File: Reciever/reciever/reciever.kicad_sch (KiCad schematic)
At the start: 24 parts, among them J1 USB_C_Receptacle_USB2.0_14P, J2 UART/I2C, J3 TWAI, SW1 Button, SW2 Button, U1 TXS0102DCU, U2 LM66200, U3 SE5218ALG-LF, U4 ESP32-C6-MINI-1, U5 TCAN330DR

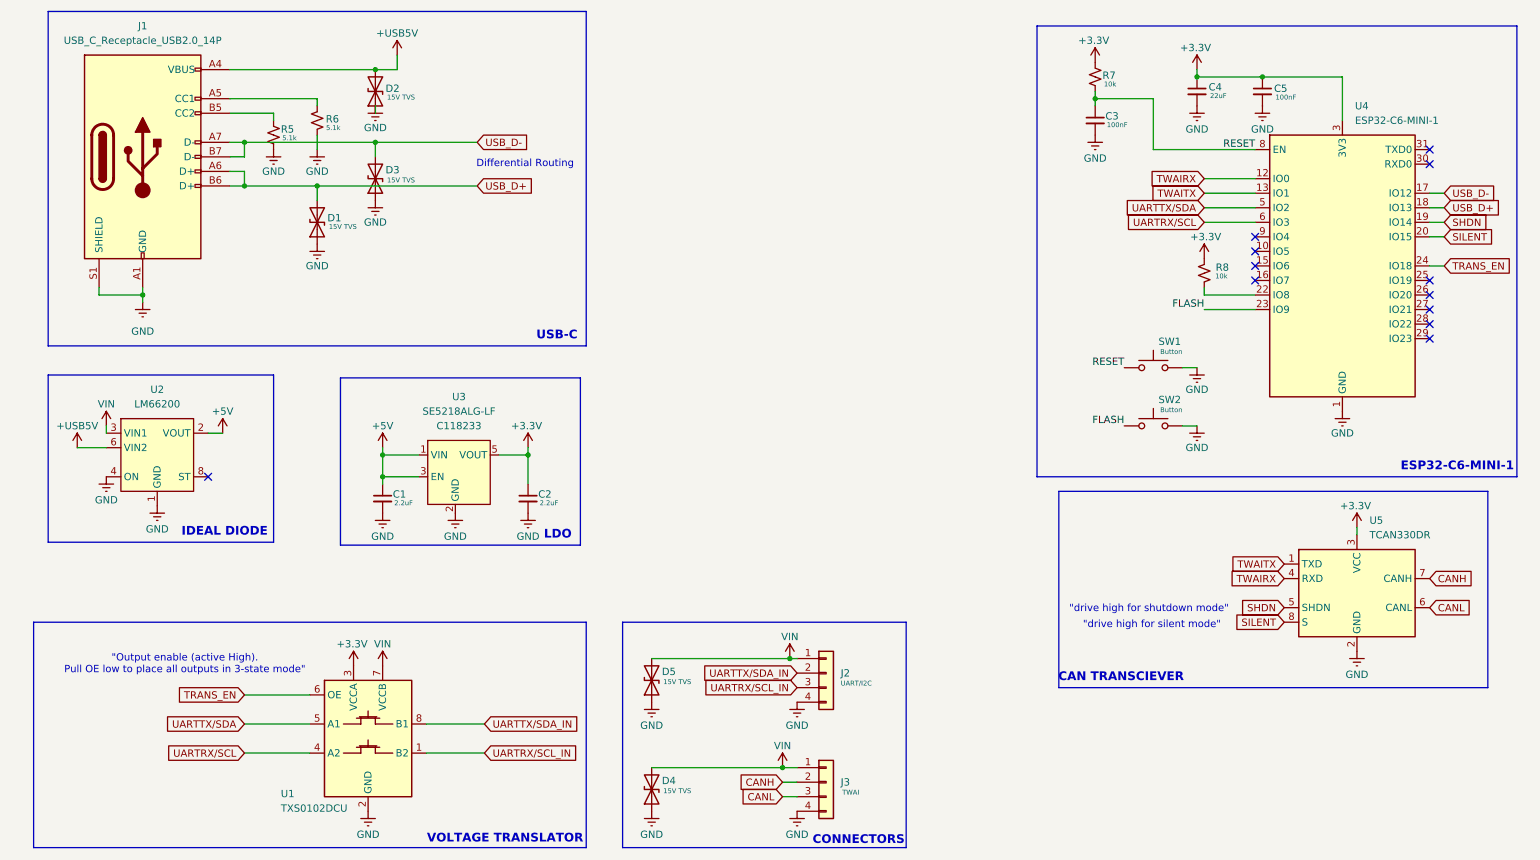
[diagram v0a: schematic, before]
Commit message: Custom RC V2
Final Remote + Receiver!

Special thanks to the CRCW25 Electrical Team who contributed to its development!

Jun
Katie
Nelson
David
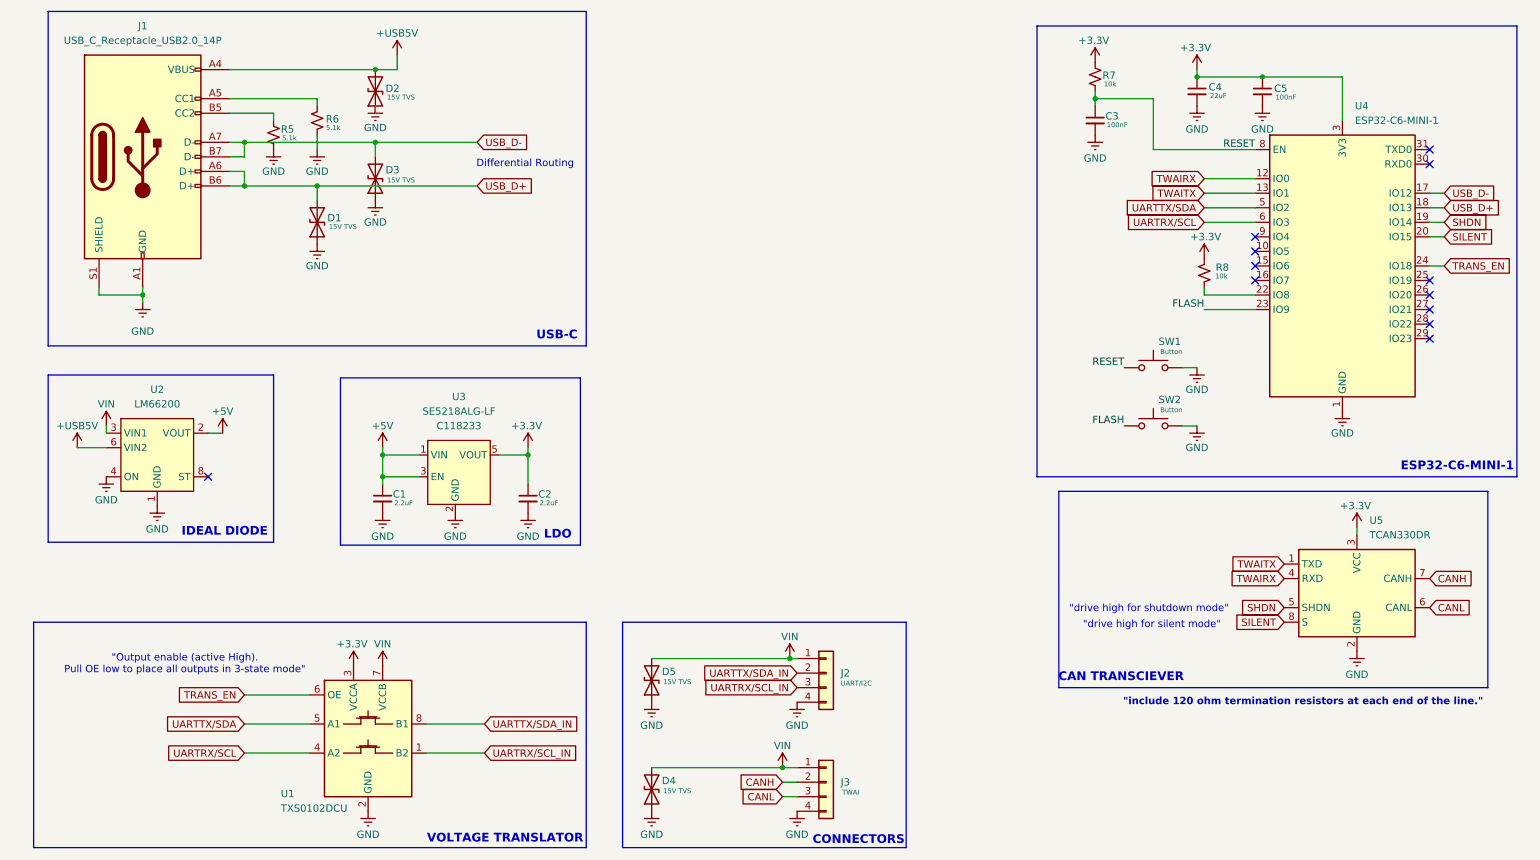
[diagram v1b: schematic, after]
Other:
- note added: ""include 120 ohm termination resistors at each end of the line.""
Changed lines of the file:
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@@
 (kicad_sch
-	(version 20231120)
+	(version 20250114)
 	(generator "eeschema")
-	(generator_version "8.0")
+	(generator_version "9.0")
 	(paper "A4")
+	(rectangle
+		(start 198.12 15.24)
+		(end 281.94 93.98)
+		(stroke
+			(width 0)
+			(type default)
+		)
+		(fill
+			(type none)
+		)
+	)
+	(rectangle
+		(start 25.4 12.7)
+		(end 119.38 71.12)
+		(stroke
+			(width 0)
+			(type default)
+		)
+		(fill
+			(type none)
+		)
+	)
+	(rectangle
+		(start 76.454 76.708)
+		(end 118.364 105.918)
+		(stroke
+			(width 0)
+			(type default)
+		)
+		(fill
+			(type none)
+		)
+	)
+	(rectangle
+		(start 22.86 119.38)
+		(end 119.38 158.75)
+		(stroke
+			(width 0)
+			(type default)
+		)
+		(fill
+			(type none)
+		)
+	)
+	(rectangle
+		(start 201.93 96.52)
+		(end 276.86 130.81)
+		(stroke
+			(width 0)
+			(type default)
+		)
+		(fill
+			(type none)
+		)
+	)
+	(rectangle
+		(start 125.73 119.38)
+		(end 175.26 158.75)
+		(stroke
+			(width 0)
+			(type default)
+		)
+		(fill
+			(type none)
+		)
+	)
+	(rectangle
+		(start 25.4 76.2)
+		(end 64.77 105.41)
+		(stroke
+			(width 0)
+			(type default)
+		)
+		(fill
+			(type none)
+		)
+	)
+	(text "\"drive high for silent mode\""
+		(exclude_from_sim no)
+		(at 218.186 119.888 0)
+		(effects
+			(font
+				(size 1.27 1.27)
+			)
+		)
+	)
+	(text "\"Output enable (active High).\nPull OE low to place all outputs in 3-state mode\""
+		(exclude_from_sim no)
+		(at 49.276 126.746 0)
+		(effects
+			(font
+				(size 1.27 1.27)
+			)
+		)
+	)
+	(text "USB-C"
+		(exclude_from_sim no)
+		(at 117.856 69.342 0)
+		(effects
+			(font
+				(face "KiCad Font")
+				(size 1.524 1.524)
+				(thickness 0.3048)
+				(bold yes)
+			)
+			(justify right)
+		)
+	)
+	(text "Differential Routing"
+		(exclude_from_sim no)
+		(at 108.712 39.37 0)
+		(effects
+			(font
+				(size 1.27 1.27)
+			)
+		)
+	)
+	(text "\"include 120 ohm termination resistors at each end of the line.\""
+		(exclude_from_sim no)
+		(at 244.602 133.35 0)
+		(effects
+			(font
+				(size 1.27 1.27)
+				(thickness 0.254)
+				(bold yes)
+			)
+		)
+	)
+	(text "VOLTAGE TRANSLATOR"
+		(exclude_from_sim no)
+		(at 118.872 157.226 0)
+		(effects
+			(font
+				(face "KiCad Font")
+				(size 1.524 1.524)
+				(thickness 0.3048)
+				(bold yes)
+			)
+			(justify right)
+		)
+	)
+	(text "CONNECTORS"
+		(exclude_from_sim no)
+		(at 175.006 157.48 0)
+		(effects
+			(font
+				(face "KiCad Font")
+				(size 1.524 1.524)
+				(thickness 0.3048)
+				(bold yes)
+			)
+			(justify right)
+		)
+	)
+	(text "\"drive high for shutdown mode\""
+		(exclude_from_sim no)
+		(at 217.678 117.094 0)
+		(effects
+			(font
+				(size 1.27 1.27)
+			)
+		)
+	)
+	(text "ESP32-C6-MINI-1"
+		(exclude_from_sim no)
+		(at 281.432 92.202 0)
+		(effects
+			(font
+				(face "KiCad Font")
+				(size 1.524 1.524)
+				(thickness 0.3048)
+				(bold yes)
+			)
+			(justify right)
+		)
+	)
+	(text "IDEAL DIODE"
+		(exclude_from_sim no)
+		(at 63.754 103.632 0)
+		(effects
+			(font
+				(face "KiCad Font")
+				(size 1.524 1.524)
+				(thickness 0.3048)
+				(bold yes)
+			)
+			(justify right)
+		)
+	)
+	(text "LDO"
+		(exclude_from_sim no)
+		(at 116.84 104.14 0)
+		(effects
+			(font
+				(face "KiCad Font")
+				(size 1.524 1.524)
+				(thickness 0.3048)
+				(bold yes)
+			)
+			(justify right)
+		)
+	)
+	(text "CAN TRANSCIEVER"
+		(exclude_from_sim no)
+		(at 223.774 129.032 0)
+		(effects
+			(font
+				(face "KiCad Font")
+				(size 1.524 1.524)
+				(thickness 0.3048)
+				(bold yes)
+			)
+			(justify right)
+		)
+	)
 	(junction
 		(at 154.94 125.73)
@@
 		)
 	)
-	(rectangle
-		(start 198.12 15.24)
-		(end 281.94 93.98)
-		(stroke
-			(width 0)
-			(type default)
-		)
-		(fill
-			(type none)
-		)
-	)
-	(rectangle
-		(start 25.4 12.7)
-		(end 119.38 71.12)
-		(stroke
-			(width 0)
-			(type default)
-		)
-		(fill
-			(type none)
-		)
-	)
-	(rectangle
-		(start 76.454 76.708)
-		(end 118.364 105.918)
-		(stroke
-			(width 0)
-			(type default)
-		)
-		(fill
-			(type none)
-		)
-	)
-	(rectangle
-		(start 22.86 119.38)
-		(end 119.38 158.75)
-		(stroke
-			(width 0)
-			(type default)
-		)
-		(fill
-			(type none)
-		)
-	)
-	(rectangle
-		(start 201.93 96.52)
-		(end 276.86 130.81)
-		(stroke
-			(width 0)
-			(type default)
-		)
-		(fill
-			(type none)
-		)
-	)
-	(rectangle
-		(start 125.73 119.38)
-		(end 175.26 158.75)
-		(stroke
-			(width 0)
-			(type default)
-		)
-		(fill
-			(type none)
-		)
-	)
-	(rectangle
-		(start 25.4 76.2)
-		(end 64.77 105.41)
-		(stroke
-			(width 0)
-			(type default)
-		)
-		(fill
-			(type none)
-		)
-	)
-	(text "\"drive high for silent mode\""
-		(exclude_from_sim no)
-		(at 218.186 119.888 0)
-		(effects
-			(font
-				(size 1.27 1.27)
-			)
-		)
-	)
-	(text "\"Output enable (active High).\nPull OE low to place all outputs in 3-state mode\""
-		(exclude_from_sim no)
-		(at 49.276 126.746 0)
-		(effects
-			(font
-				(size 1.27 1.27)
-			)
-		)
-	)
-	(text "USB-C"
-		(exclude_from_sim no)
-		(at 117.856 69.342 0)
-		(effects
-			(font
-				(face "KiCad Font")
-				(size 1.524 1.524)
-				(thickness 0.3048)
-				(bold yes)
-			)
-			(justify right)
-		)
-	)
-	(text "Differential Routing"
-		(exclude_from_sim no)
-		(at 108.712 39.37 0)
-		(effects
-			(font
-				(size 1.27 1.27)
-			)
-		)
-	)
-	(text "VOLTAGE TRANSLATOR"
-		(exclude_from_sim no)
-		(at 118.872 157.226 0)
-		(effects
-			(font
-				(face "KiCad Font")
-				(size 1.524 1.524)
-				(thickness 0.3048)
-				(bold yes)
-			)
-			(justify right)
-		)
-	)
-	(text "CONNECTORS"
-		(exclude_from_sim no)
-		(at 175.006 157.48 0)
-		(effects
-			(font
-				(face "KiCad Font")
-				(size 1.524 1.524)
-				(thickness 0.3048)
-				(bold yes)
-			)
-			(justify right)
-		)
-	)
-	(text "\"drive high for shutdown mode\""
-		(exclude_from_sim no)
-		(at 217.678 117.094 0)
-		(effects
-			(font
-				(size 1.27 1.27)
-			)
-		)
-	)
-	(text "ESP32-C6-MINI-1"
-		(exclude_from_sim no)
-		(at 281.432 92.202 0)
-		(effects
-			(font
-				(face "KiCad Font")
-				(size 1.524 1.524)
-				(thickness 0.3048)
-				(bold yes)
-			)
-			(justify right)
-		)
-	)
-	(text "IDEAL DIODE"
-		(exclude_from_sim no)
-		(at 63.754 103.632 0)
-		(effects
-			(font
-				(face "KiCad Font")
-				(size 1.524 1.524)
-				(thickness 0.3048)
-				(bold yes)
-			)
-			(justify right)
-		)
-	)
-	(text "LDO"
-		(exclude_from_sim no)
-		(at 116.84 104.14 0)
-		(effects
-			(font
-				(face "KiCad Font")
-				(size 1.524 1.524)
-				(thickness 0.3048)
-				(bold yes)
-			)
-			(justify right)
-		)
-	)
-	(text "CAN TRANSCIEVER"
-		(exclude_from_sim no)
-		(at 223.774 129.032 0)
-		(effects
-			(font
-				(face "KiCad Font")
-				(size 1.524 1.524)
-				(thickness 0.3048)
-				(bold yes)
-			)
-			(justify right)
-		)
-	)
 	(label "FLASH"
 		(at 213.36 85.09 180)
@@
 		)
 	)
+	(embedded_fonts no)
 )
